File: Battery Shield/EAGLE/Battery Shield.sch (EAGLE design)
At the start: 31 parts, among them IC1 MCP73871, U1 TPS61200

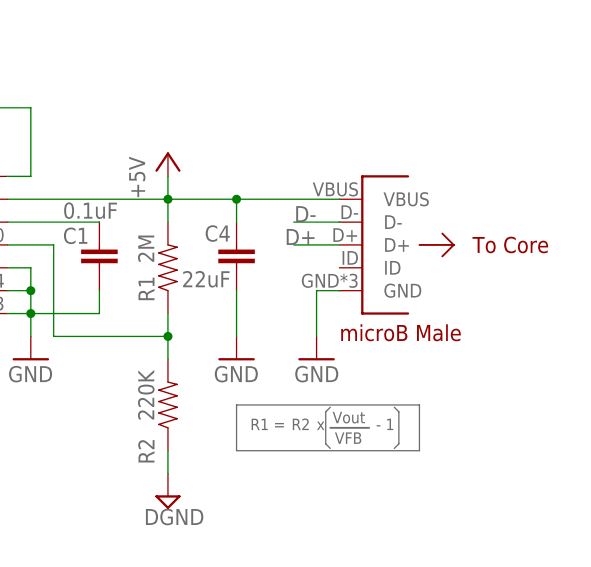
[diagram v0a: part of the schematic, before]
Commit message: updated battery shield
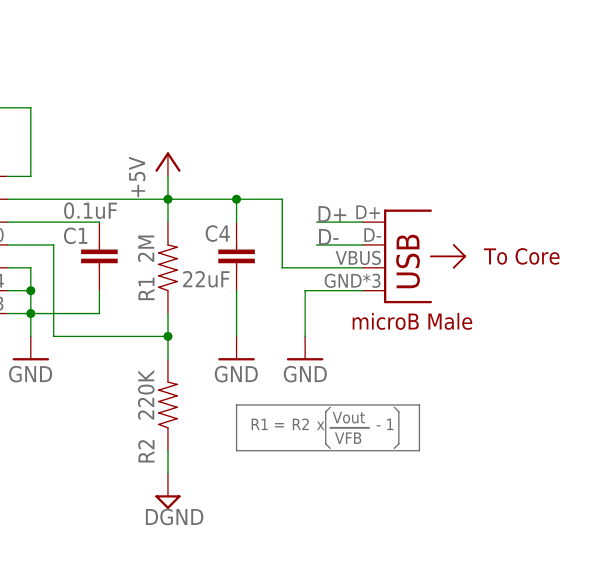
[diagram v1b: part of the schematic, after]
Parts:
- removed U$1: USB_MALE, Spark:USB_MALE
- added JP2: USBFCI, Spark:USBFCI
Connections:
- net +5V: now also JP2.VBUS; no longer U$1.VBUS
- net D+: now also JP2.D+; no longer U$1.D+
- net D-: now also JP2.D-; no longer U$1.D-
- net GND: now also JP2.GND; no longer U$1.GND
